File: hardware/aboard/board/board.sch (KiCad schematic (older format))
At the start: 19 parts, among them P1 Power, P2 Analog, P3 Digital, P4 Digital, P5 CONN_01X01, P6 CONN_01X01, P7 CONN_01X01, P8 CONN_01X01, U1 24LC512, U10 ST25DV04K, U11 ST25DV04K, U2 AT25SF081-SSHD-X, U3 24LC512, U4 AT25SF081-SSHD-X, U5 24LC512, U6 LTC3406ES5, U7 LTC3406ES5, U8 Si5351A, U9 ICE40UP5K-SG48ITR

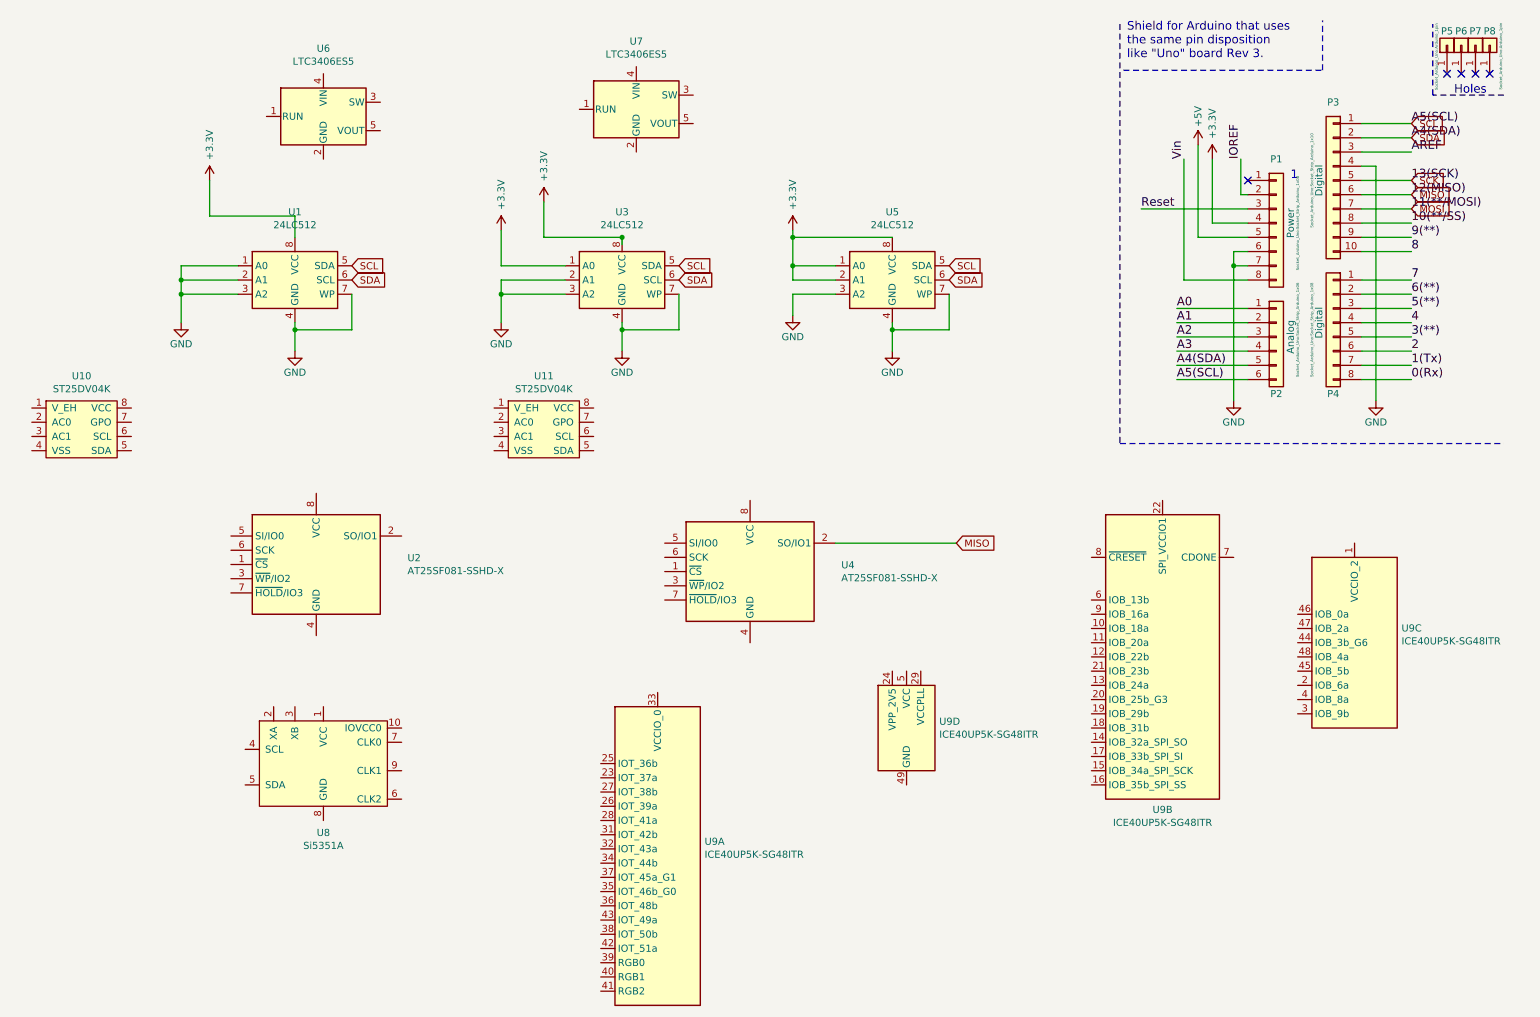
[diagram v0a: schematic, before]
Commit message: board for OM13088UL: process 1
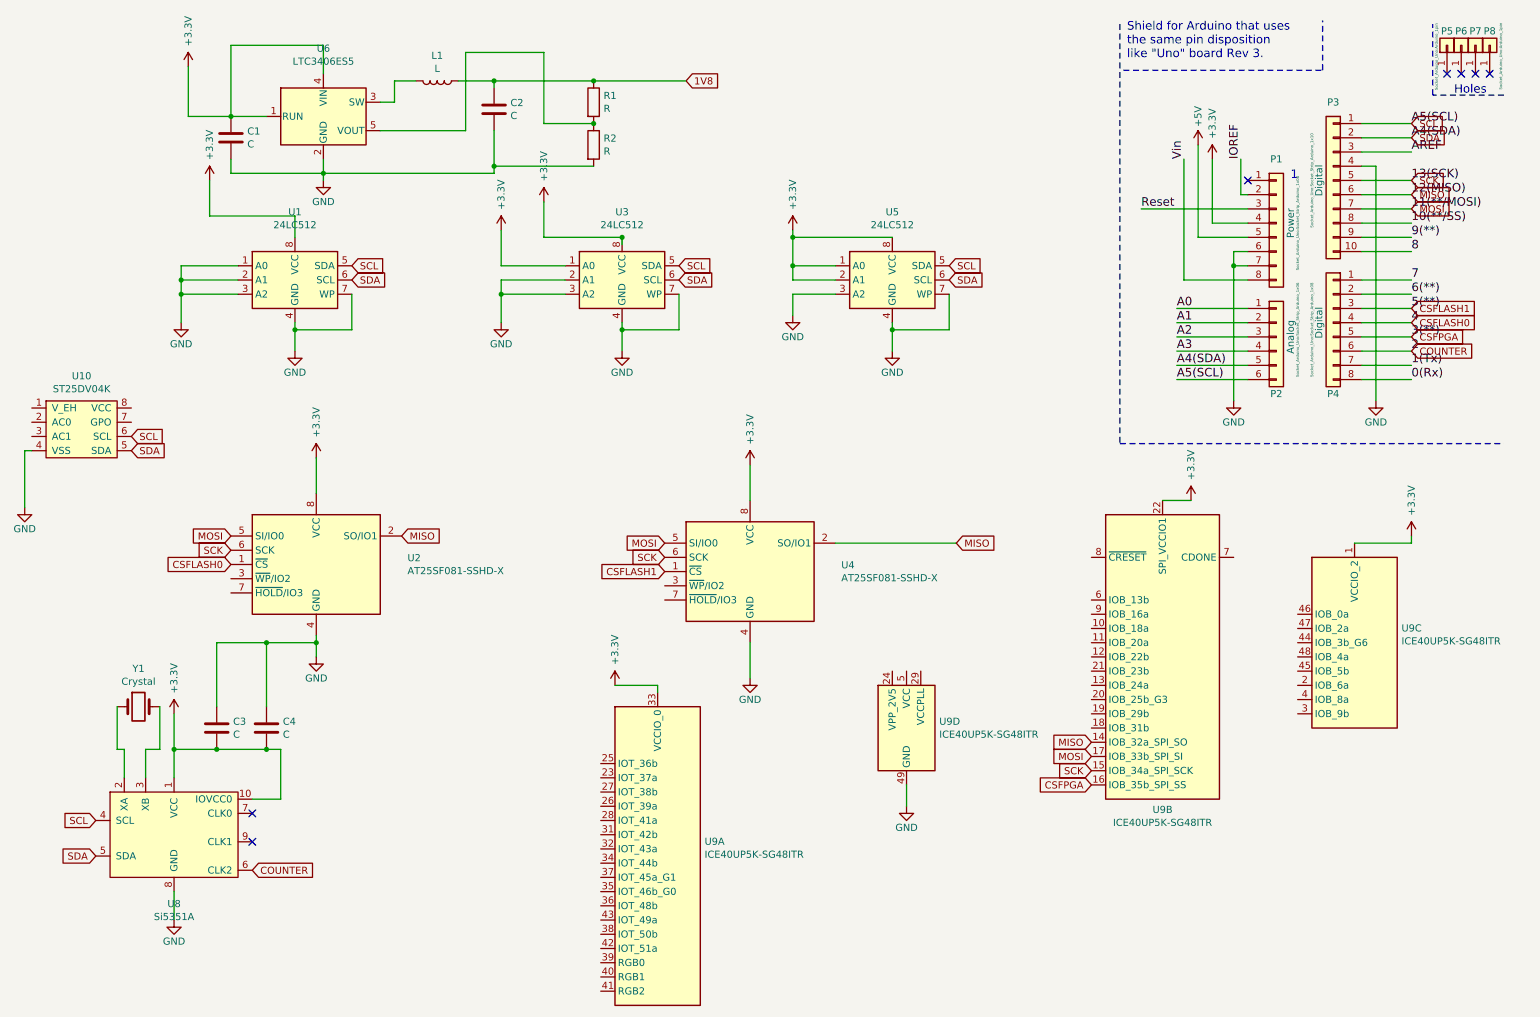
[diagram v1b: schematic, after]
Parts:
- removed U11: ST25DV04K, symbol kilib:ST25DV04K
- removed U7: LTC3406ES5, Package_TO_SOT_SMD:TSOT-23-5, symbol Regulator_Switching:LTC3406ES5
- added C1, C2, C3, C4: C, symbol Device:C
- added L1: L, symbol Device:L
- added R1, R2: R, symbol Device:R
- added Y1: Crystal, symbol Device:Crystal
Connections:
- net 2 is gone; now on net COUNTER: P4.6 (Pin_6)
- net 3(**) is gone; now on net CSFPGA: P4.5 (Pin_5)
- net 4 is gone; now on net CSFLASH0: P4.4 (Pin_4)
- net 5(**) is gone; now on net CSFLASH1: P4.3 (Pin_3)
- net +3V3: now also U2.8 (VCC), U4.8 (VCC), U6.1 (RUN), U6.4 (VIN), U8.1 (VCC), U8.10 (IOVCC0), U9.1 (VCCIO_2), U9.22 (SPI_VCCIO1), U9.33 (VCCIO_0), C1.1, C3.2, C4.2
- net GND: now also U10.4 (VSS), U2.4 (GND), U4.4 (GND), U6.2 (GND), U8.8 (GND), U9.49 (GND), C1.2, C2.2, C3.1, C4.1, R2.2
- net MISO: now also U2.2 (SO/IO1), U9.14 (IOB_32a_SPI_SO)
- net MOSI: now also U2.5 (SI/IO0), U4.5 (SI/IO0), U9.17 (IOB_33b_SPI_SI)
- net SCK: now also U2.6 (SCK), U4.6 (SCK), U9.15 (IOB_34a_SPI_SCK)
- net SCL: now also U10.6 (SCL), U8.4 (SCL)
- net SDA: now also U10.5 (SDA), U8.5 (SDA)
- net CSFLASH0: now reaches U2.1 (~CS)
- net CSFLASH1: now reaches U4.1 (~CS)
- net at U6.3 (SW): now also L1.2
- net at U6.5 (VOUT): now also R1.2, R2.1
- net at U8.2 (XA): now also Y1.1
- net at U8.3 (XB): now also Y1.2
- net COUNTER: now reaches U8.6 (CLK2)
- net CSFPGA: now reaches U9.16 (IOB_35b_SPI_SS)
- new net 1V8: C2.1, L1.1, R1.1
- no-connect marks 5 -> 7
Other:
- moved on the sheet: U8
